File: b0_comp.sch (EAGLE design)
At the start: 273 parts, among them IC1 КР1006ВИ1(NE555), IC3 LM358D, IC4 78L09F, IC6 MEGA8-AI, IC7 74121N, IC8 4030N, IC9 LM324D, T1P T90, -26 MicroMetals Yellow-W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

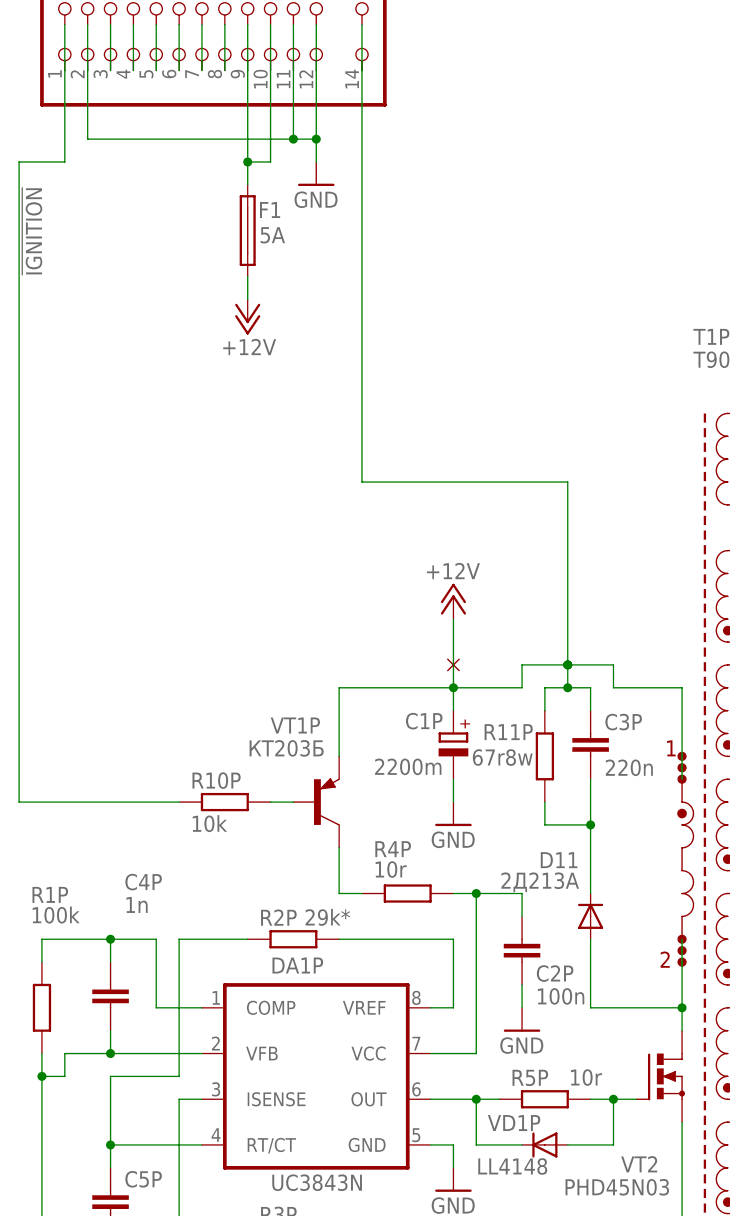
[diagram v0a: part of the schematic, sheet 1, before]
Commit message: .
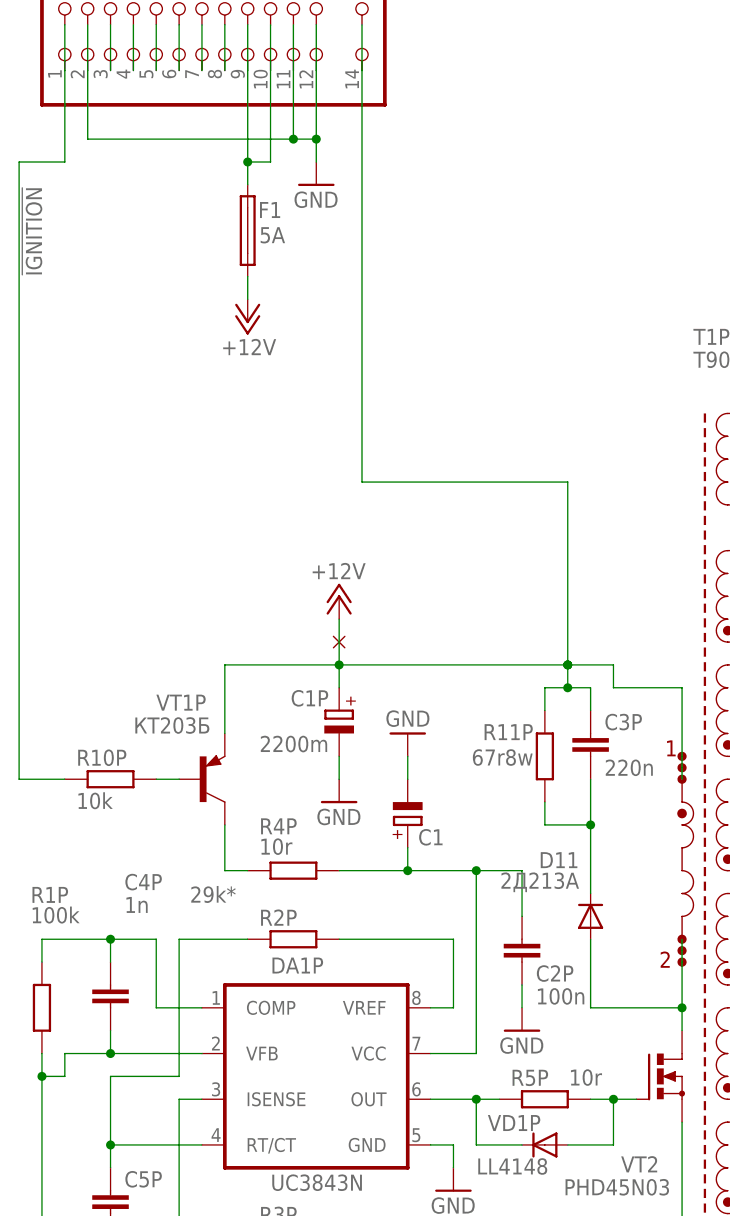
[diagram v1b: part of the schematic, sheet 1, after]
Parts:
- added C1: (no value), rcl:CPOL-EUE2.5-5
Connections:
- net GND: now also C1.-
- net N$30: now also C1.+
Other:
- moved on the sheet: C1P, R10P, R4P, VT1P
